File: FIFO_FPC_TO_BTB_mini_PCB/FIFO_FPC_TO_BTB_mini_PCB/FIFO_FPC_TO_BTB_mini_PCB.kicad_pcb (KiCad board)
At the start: 4 copper layers, 83.5 x 61.5 mm, 2 parts, among them J1 SFV30R-1STE1HLF, J2 DF40C_2.0_-60DS-0.4V_51_

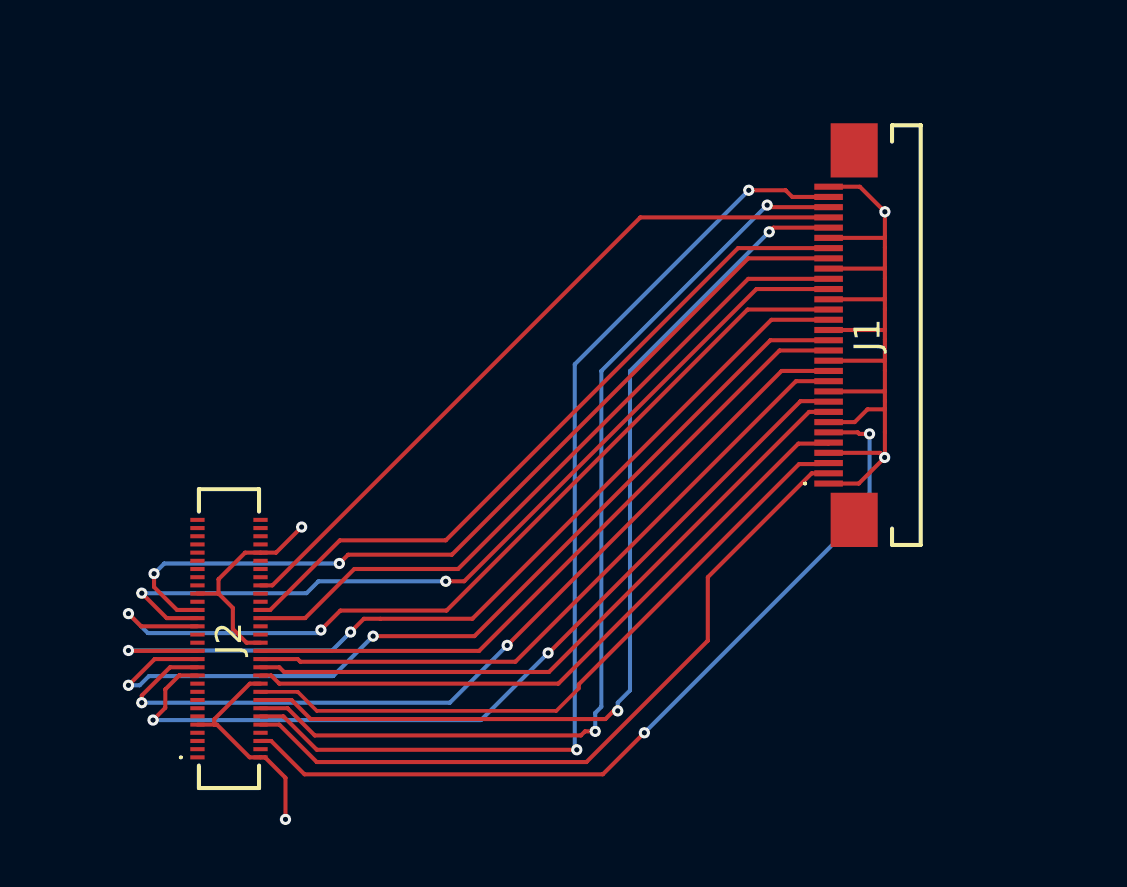
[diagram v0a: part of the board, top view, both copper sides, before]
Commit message: w
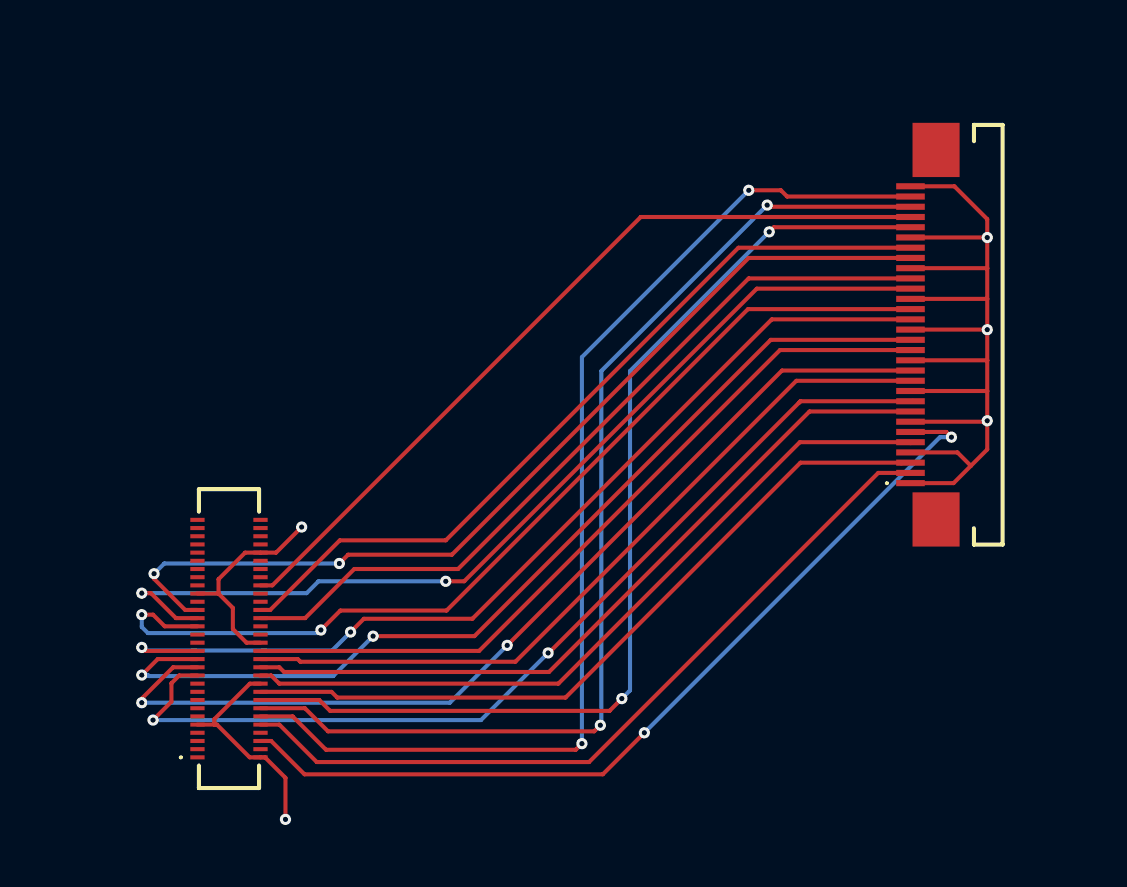
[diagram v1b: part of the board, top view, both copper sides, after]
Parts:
- moved J1 4.00 mm to (155.3, 99.3)
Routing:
- net GND: track 62.1 -> 70.7 mm, vias 4 -> 5
- net /Hed_DSP_Q0: track 32.8 -> 36.8 mm
- net /Hed_Read_CLK: track 35.2 -> 39.2 mm
- net /Hed_DSP_Q4: track 33.5 -> 37.5 mm
- net /Hed_DSP_Q2: track 33.1 -> 37.1 mm
- net /hed_DSP_Q6: track 33.8 -> 37.8 mm
- net /Hed_DSP_Q11: track 35.1 -> 39.1 mm
- net /hed_DSP_Q9: track 34.6 -> 38.6 mm
- net /hed_DSP_Q10: track 42.9 -> 46.9 mm
- net /Hed_DSP_Q1: track 43.3 -> 47.3 mm
- net /hed_~{Write_enable}: track 49.2 -> 53.1 mm
- net /Hed_DSP_Q3: track 43.9 -> 47.8 mm
- net /Hed_OUTPUT_ENABLE: track 51.1 -> 54.9 mm
- net /~{Hed_Empty_flag}_Output: track 33.3 -> 37.1 mm
- net /hed_DSP_Q12: track 42.6 -> 46.3 mm
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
